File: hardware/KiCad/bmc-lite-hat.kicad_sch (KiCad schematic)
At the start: 5 parts, among them J1 Conn_02x20_Odd_Even, SW1_XIAO-POWER-ISOLATION DEV - RUN, U1 XIAO-RP2040-DIP, U2 MCP23008-xSS

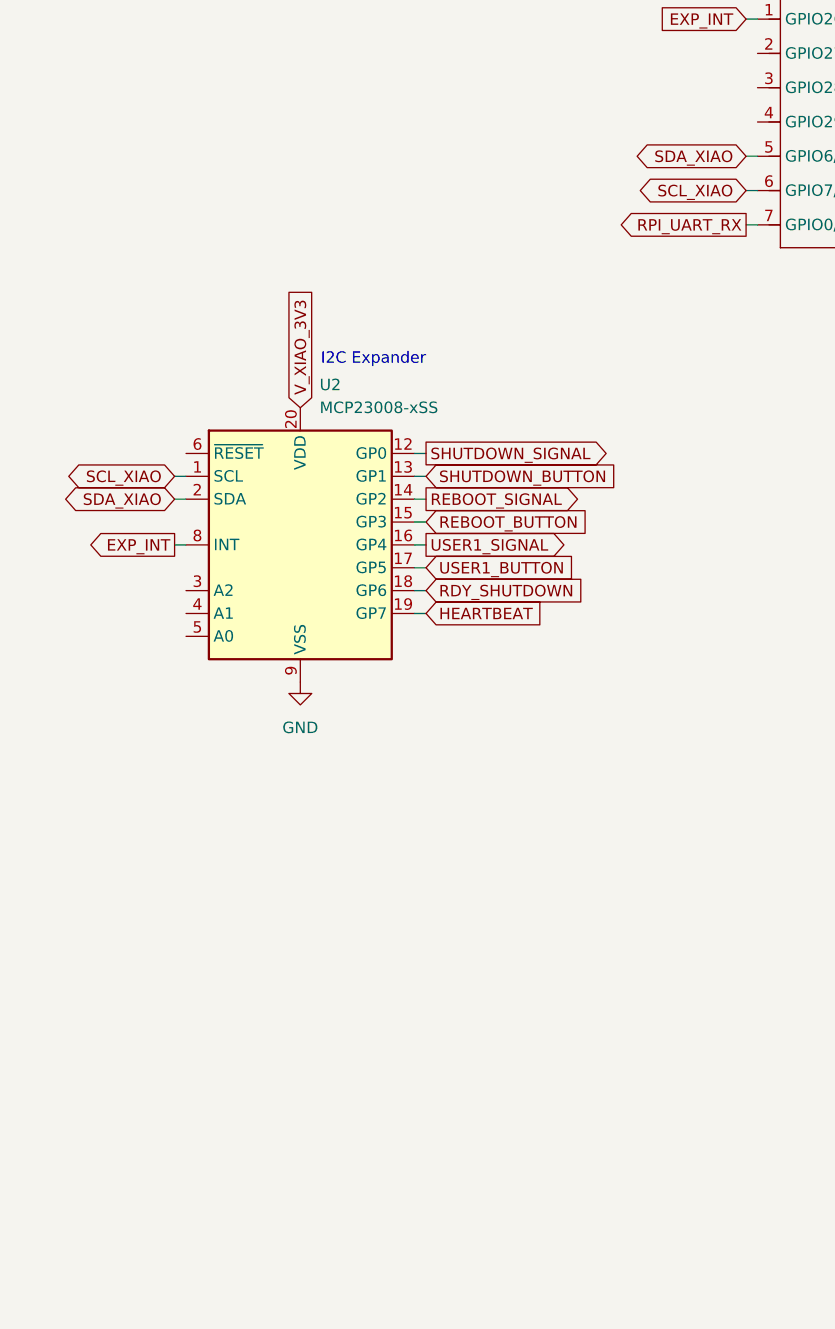
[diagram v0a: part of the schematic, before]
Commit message: Update hardware files
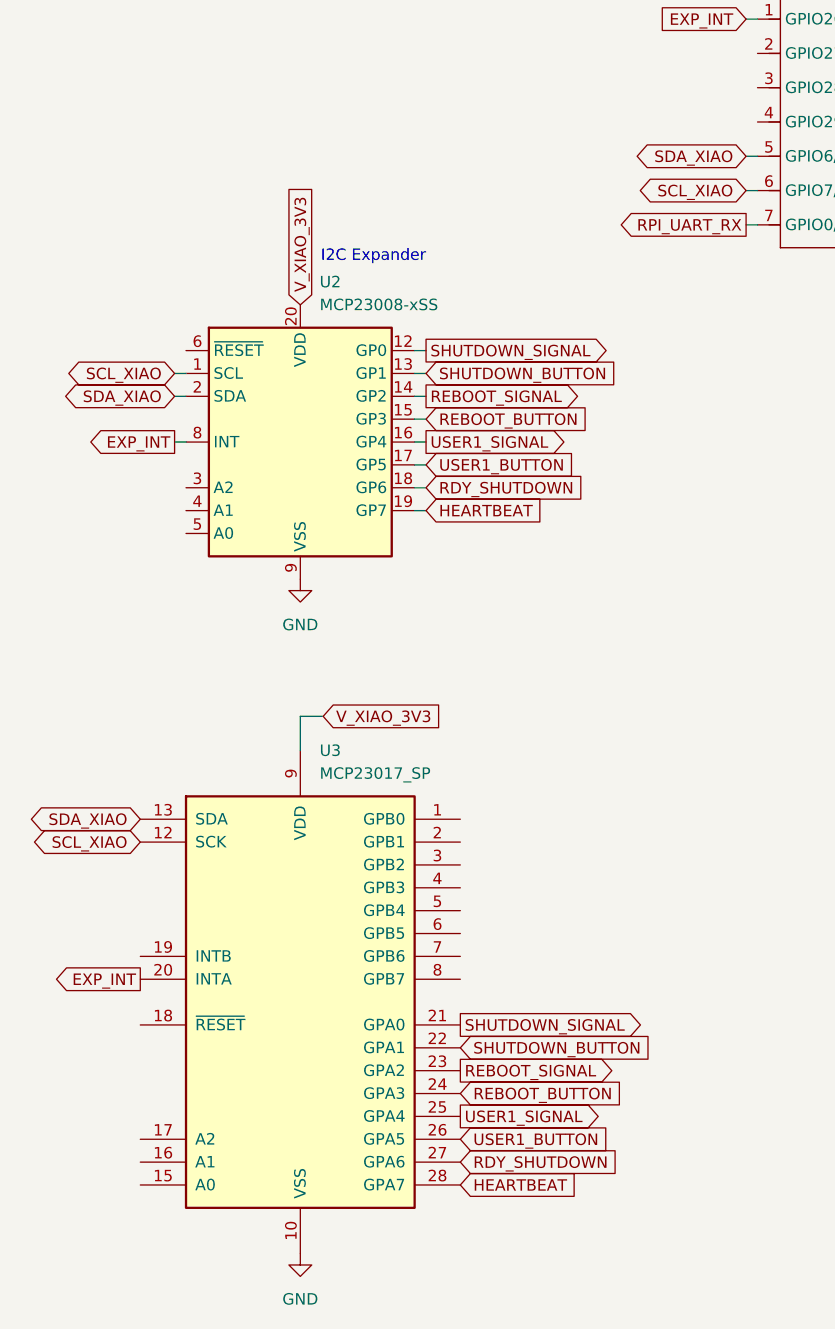
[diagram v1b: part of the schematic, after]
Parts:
- added U3: MCP23017_SP, Package_DIP:DIP-28_W7.62mm, symbol Interface_Expansion:MCP23017_SP
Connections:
- net EXP_INT: now also U3.20 (INTA)
- net GND: now also U3.10 (VSS)
- net HEARTBEAT: now also U3.28 (GPA7)
- net RDY_SHUTDOWN: now also U3.27 (GPA6)
- net REBOOT_BUTTON: now also U3.24 (GPA3)
- net REBOOT_SIGNAL: now also U3.23 (GPA2)
- net SCL_XIAO: now also U3.12 (SCK)
- net SDA_XIAO: now also U3.13 (SDA)
- net SHUTDOWN_BUTTON: now also U3.22 (GPA1)
- net SHUTDOWN_SIGNAL: now also U3.21 (GPA0)
- net USER1_BUTTON: now also U3.26 (GPA5)
- net USER1_SIGNAL: now also U3.25 (GPA4)
- net V_XIAO_3V3: now also U3.9 (VDD)
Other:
- moved on the sheet: U2
